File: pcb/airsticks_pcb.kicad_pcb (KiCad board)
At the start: 2 copper layers, 66.5 x 22.5 mm, 17 parts, among them J1 USB_C_Receptacle_USB2.0, J2 STM_LINK, J3 USB_SERIAL_TTL, J4 I2C, J5 AudioJack3, U1 STM32G441KBT6, U4 PAM8302AAS, U5 TC1262-33

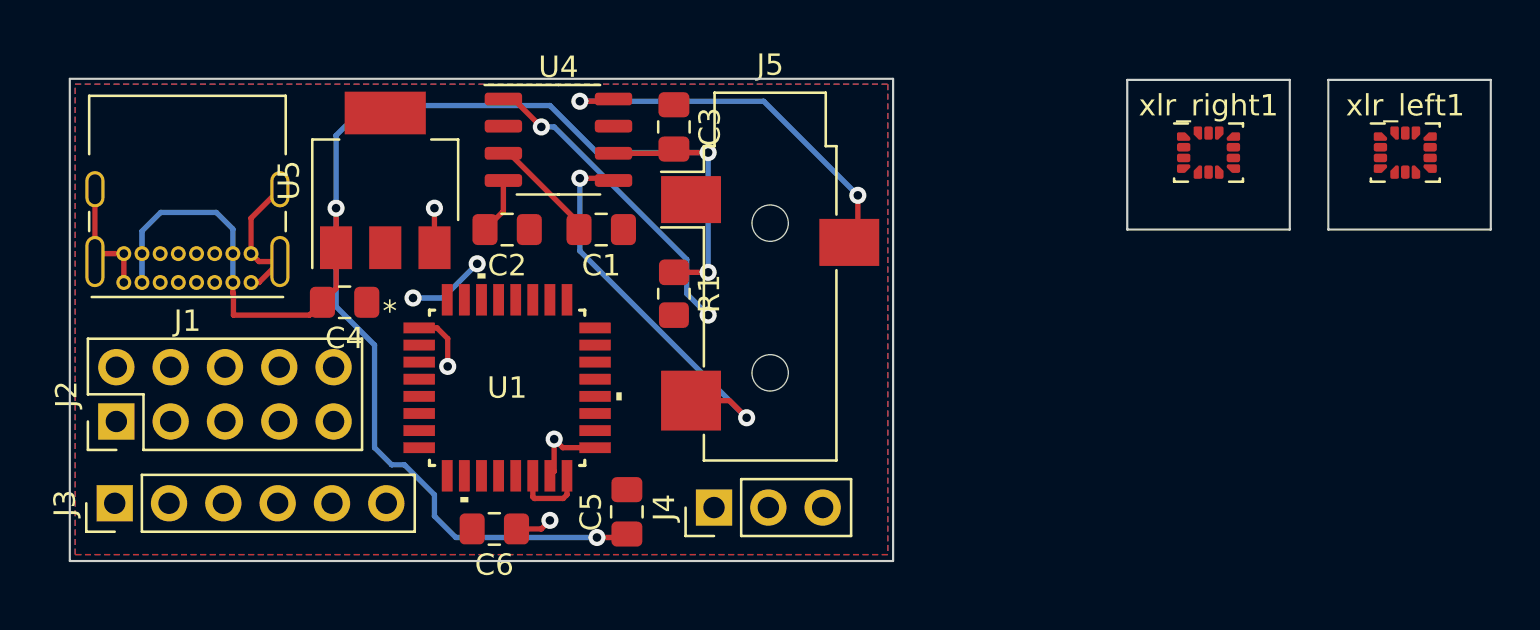
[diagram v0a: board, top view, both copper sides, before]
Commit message: finished pcb
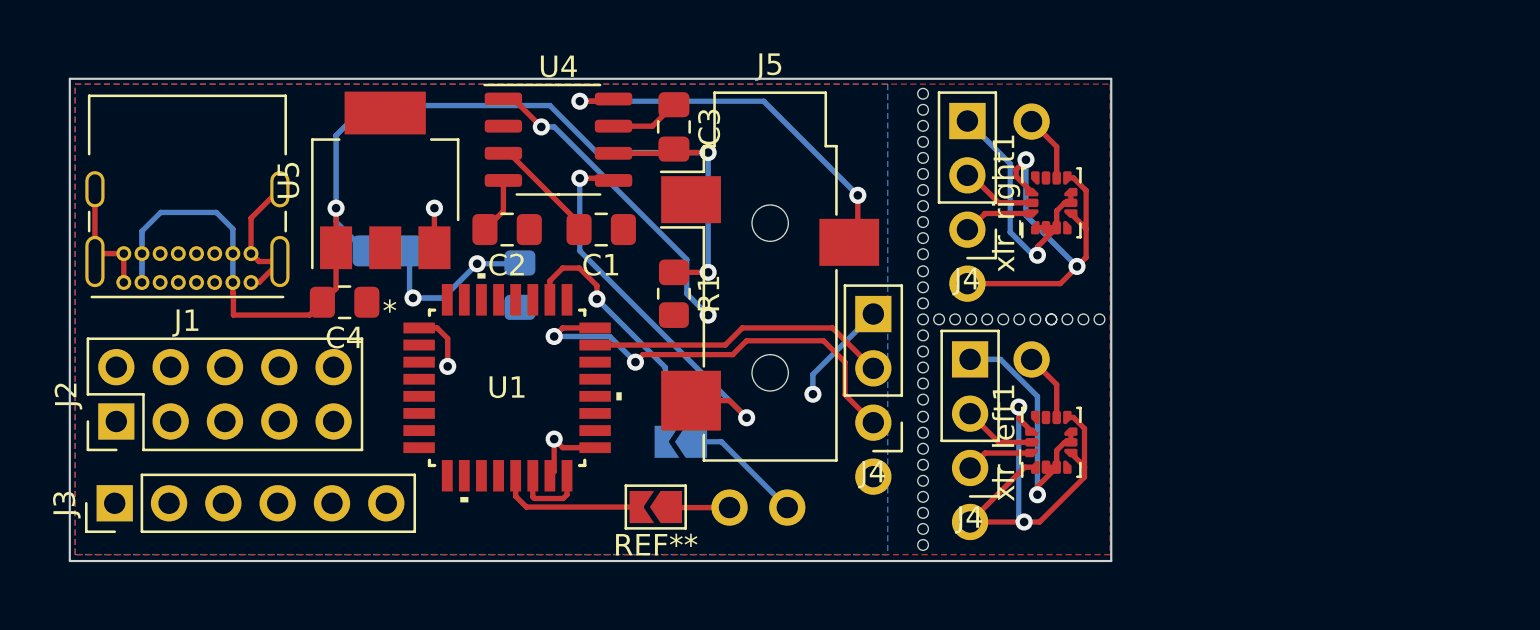
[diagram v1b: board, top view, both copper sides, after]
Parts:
- removed the J4 at (49.9, 73.8)
- added ?: , , F.Cu at (59.6, 67.2)
- added ?: , , F.Cu at (59.6, 56.0)
- added ?: , , F.Cu at (64.9, 65.0)
- added ?: , , F.Cu at (59.6, 59.7)
- added ?: , , F.Cu at (59.6, 65.8)
- added ?: , , F.Cu at (64.2, 65.0)
- added ?: , , F.Cu at (59.6, 56.7)
- added ?: , , F.Cu at (59.6, 57.5)
- added ?: , , F.Cu at (59.6, 75.5)
- added ?: , , F.Cu at (59.6, 62.8)
- added ?: , , F.Cu at (59.6, 68.8)
- added ?: , , F.Cu at (57.3, 72.4)
- added ?: , , F.Cu at (59.6, 64.2)
- added ?: , , F.Cu at (61.9, 74.5)
- added ?: , , F.Cu at (59.6, 71.0)
- added ? (x2): , , F.Cu at (65.7, 65.0)
- added ?: , , F.Cu at (59.6, 73.3)
- added ?: , , F.Cu at (59.6, 69.5)
- added ?: , , F.Cu at (59.6, 63.5)
- added ?: , , F.Cu at (59.6, 59.0)
- added ?: , , F.Cu at (59.6, 65.0)
- added ?: , , F.Cu at (67.2, 65.0)
- added ?: , , F.Cu at (62.6, 65.0)
- added ?: , , F.Cu at (63.4, 65.0)
- added ?: , , F.Cu at (64.7, 55.8)
- added ?: , , F.Cu at (59.6, 74.8)
- added ?: , , F.Cu at (59.6, 55.2)
- added ?: , , F.Cu at (59.6, 72.5)
- added ?: , , F.Cu at (53.3, 73.8)
- added ?: , , F.Cu at (61.1, 65.0)
- added ?: , , F.Cu at (59.6, 62.0)
- added ?: , , F.Cu at (59.6, 61.2)
- added ?: , , F.Cu at (59.6, 68.0)
- added ?: , , F.Cu at (59.6, 70.3)
- added ?: , , F.Cu at (59.6, 66.5)
- added ?: , , F.Cu at (61.7, 63.3)
- added ?: , , F.Cu at (64.7, 66.9)
- added ?: , , F.Cu at (60.4, 65.0)
- added ?: , , F.Cu at (50.6, 73.8)
- added ?: , , F.Cu at (59.6, 58.2)
- added ?: , , F.Cu at (67.9, 65.0)
- added ?: , , F.Cu at (59.6, 60.5)
- added ?: , , F.Cu at (59.6, 74.0)
- added ?: , , F.Cu at (59.6, 71.8)
- added ?: , , F.Cu at (59.6, 54.5)
- added ?: , , F.Cu at (66.4, 65.0)
- added ?: , , F.Cu at (61.9, 65.0)
- added J4: I2C, Connector_PinHeader_2.54mm:PinHeader_1x03_P2.54mm_Vertical, F.Cu at (57.3, 69.8)
- added J4: I2C, Connector_PinHeader_2.54mm:PinHeader_1x03_P2.54mm_Vertical, F.Cu at (61.9, 72.0)
- added J4: I2C, Connector_PinHeader_2.54mm:PinHeader_1x03_P2.54mm_Vertical, F.Cu at (61.7, 60.8)
- added REF**: SolderJumper-2_P1.3mm_Open_TrianglePad1.0x1.5mm, Jumper:SolderJumper-2_P1.3mm_Open_TrianglePad1.0x1.5mm, F.Cu at (47.1, 73.8)
- added REF**: SolderJumper-2_P1.3mm_Open_TrianglePad1.0x1.5mm, Jumper:SolderJumper-2_P1.3mm_Open_TrianglePad1.0x1.5mm, B.Cu at (48.3, 70.7)
- C5, C6: moved to B.Cu
- moved xlr_left1 21.4 mm to (65.7, 70.8), turned to 90 degrees
- moved C5 16.6 mm to (34.6, 61.8), turned to 0 degrees
- moved C6 11.5 mm to (40.8, 63.4), turned to 90 degrees
- moved xlr_right1 7.72 mm to (65.7, 59.5), turned to 90 degrees
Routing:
- net +3V3: track 10.3 -> 48.9 mm, vias 4 -> 7
- net GND: track 20.3 -> 58.0 mm, vias 2 -> 5
- net /I2C1_SDA: track 0.00 -> 26.9 mm, vias 0 -> 2
- net +5V: track 80.6 -> 57.1 mm, vias 4 -> 3
- net /ACC_INT1: track 0.00 -> 21.5 mm, vias 0 -> 1
- net /I2C1_SLC: track 0.00 -> 21.1 mm
- net /ACC_INT0: track 0.00 -> 12.9 mm
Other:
- board size 66.5 x 22.5 mm -> 48.7 x 22.5 mm

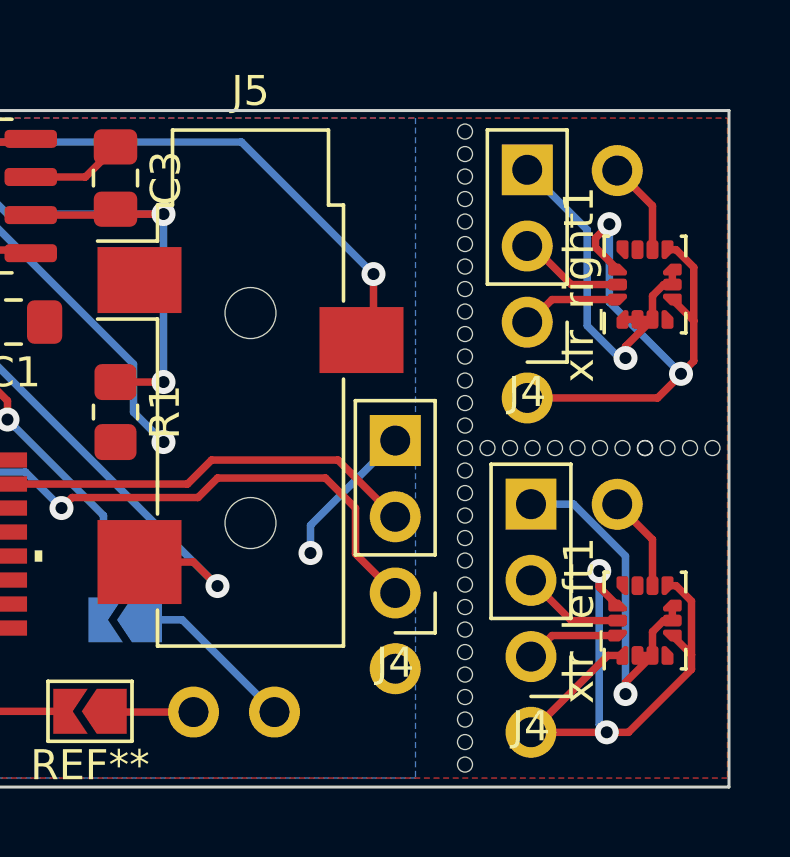
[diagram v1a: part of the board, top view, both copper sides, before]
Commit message: small changes to final pcb layout
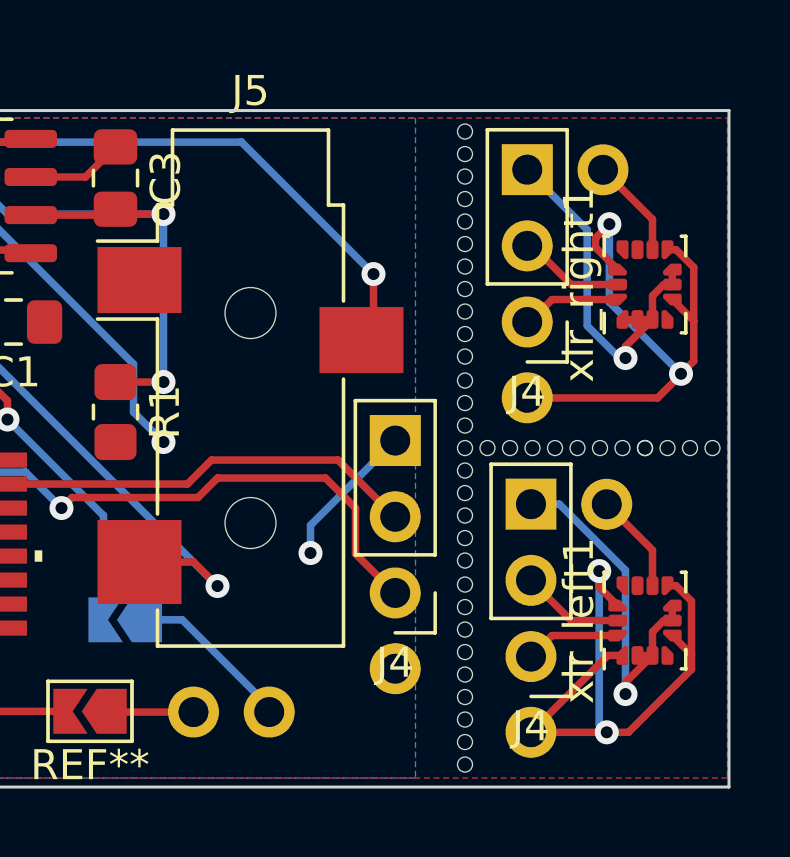
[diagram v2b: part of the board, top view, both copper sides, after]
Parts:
- removed the ? at (64.7, 55.8)
- removed the ? at (61.7, 63.3)
- added ?: , , F.Cu at (61.7, 63.3)
- added ?: , , F.Cu at (64.2, 55.7)
- moved ? 0.35 mm to (64.4, 66.9)
- moved ? 0.17 mm to (53.1, 73.8)
